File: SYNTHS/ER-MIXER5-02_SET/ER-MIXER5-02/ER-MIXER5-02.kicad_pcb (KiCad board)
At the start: 2 copper layers, 28 x 111.5 mm, 30 parts, among them J1 PJ-398SM, J2 PJ-398SM, J3 PJ-398SM, J4 PJ-398SM, J5 PJ-398SM, J6 PJ-398SM, J8 Conn_02x05, U1 TL072

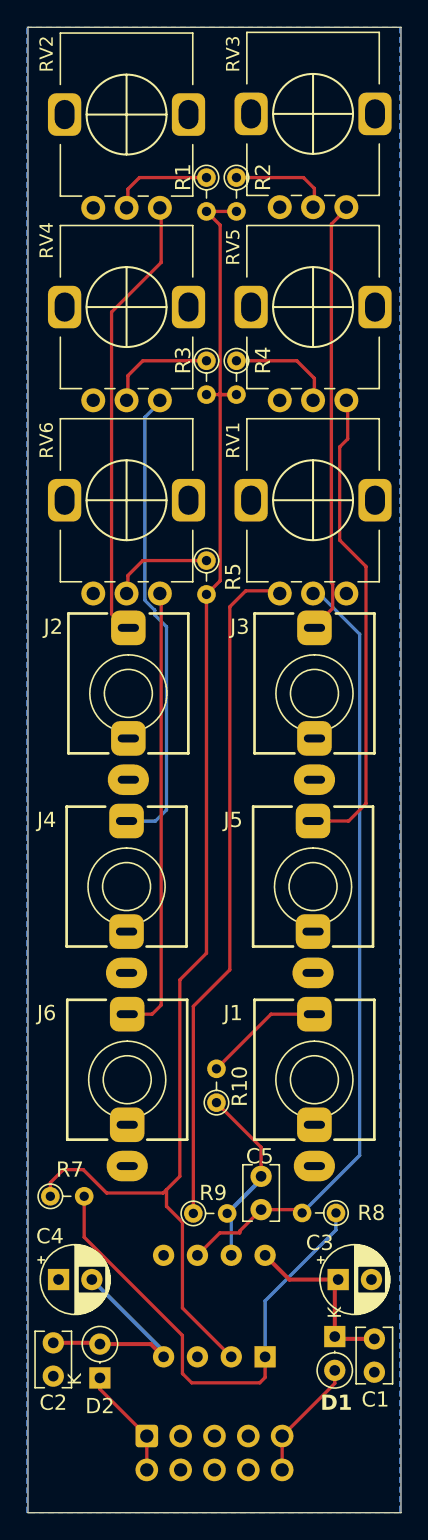
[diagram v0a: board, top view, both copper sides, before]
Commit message: cards
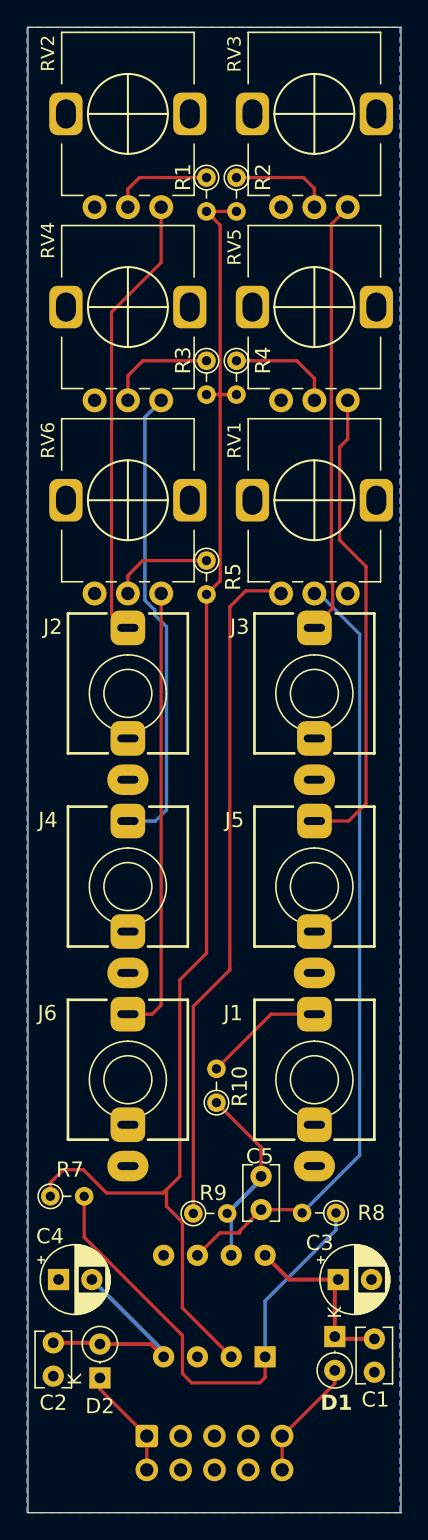
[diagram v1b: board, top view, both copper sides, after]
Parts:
- moved RV2 0.11 mm to (8.60, 15.0)
- moved J5 0.10 mm to (22.6, 73.0)
- moved RV1 0.10 mm to (22.6, 44.0)
- moved RV3 0.10 mm to (22.6, 15.0)
- moved RV5 0.10 mm to (22.6, 29.5)
- moved J4 0.10 mm to (8.60, 73.0)
- moved RV4 0.10 mm to (8.60, 29.5)
- moved RV6 0.10 mm to (8.60, 44.0)
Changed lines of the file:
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@@
   (net 23 "Net-(D2-K)")
   (footprint "LandBoards_Conns:RV09ACF" (layer "F.Cu")
-    (at 22.5 29.5 90)
+    (at 22.6 29.5 90)
     (descr "Potentiometer, vertical, Bourns PTV09A-1 Single, http://www.bourns.com/docs/Product-Datasheets/ptv09.pdf")
     (tags "Potentiometer vertical Bourns PTV09A-1 Single")
@@
   )
   (footprint "LandBoards_Conns:RV09ACF" (layer "F.Cu")
-    (at 22.5 44 90)
+    (at 22.6 44 90)
     (descr "Potentiometer, vertical, Bourns PTV09A-1 Single, http://www.bourns.com/docs/Product-Datasheets/ptv09.pdf")
     (tags "Potentiometer vertical Bourns PTV09A-1 Single")
@@
   )
   (footprint "LandBoards_Conns:RV09ACF" (layer "F.Cu")
-    (at 22.5 15 90)
+    (at 22.6 15 90)
     (descr "Potentiometer, vertical, Bourns PTV09A-1 Single, http://www.bourns.com/docs/Product-Datasheets/ptv09.pdf")
     (tags "Potentiometer vertical Bourns PTV09A-1 Single")
@@
   )
   (footprint "LandBoards_Conns:RV09ACF" (layer "F.Cu")
-    (at 8.5 44 90)
+    (at 8.6 44 90)
     (descr "Potentiometer, vertical, Bourns PTV09A-1 Single, http://www.bourns.com/docs/Product-Datasheets/ptv09.pdf")
     (tags "Potentiometer vertical Bourns PTV09A-1 Single")
@@
   )
   (footprint "AudioJacks:Jack_3.5mm_QingPu_WQP-PJ398SM_Vertical" (layer "F.Cu")
-    (at 22.5 73)
+    (at 22.6 73)
     (descr "T-S-SN Vertical mount jack AKA WQP-WQP518MA or Thonkiconn")
     (tags "WQP-WQP518MA, Thonkiconn")
@@
   )
   (footprint "AudioJacks:Jack_3.5mm_QingPu_WQP-PJ398SM_Vertical" (layer "F.Cu")
-    (at 8.55 87.5)
+    (at 8.6 87.5)
     (descr "T-S-SN Vertical mount jack AKA WQP-WQP518MA or Thonkiconn")
     (tags "WQP-WQP518MA, Thonkiconn")
@@
   )
   (footprint "AudioJacks:Jack_3.5mm_QingPu_WQP-PJ398SM_Vertical" (layer "F.Cu")
-    (at 8.636 58.5)
+    (at 8.6 58.5)
     (descr "T-S-SN Vertical mount jack AKA WQP-WQP518MA or Thonkiconn")
     (tags "WQP-WQP518MA, Thonkiconn")
@@
   )
   (footprint "AudioJacks:Jack_3.5mm_QingPu_WQP-PJ398SM_Vertical" (layer "F.Cu")
-    (at 8.5 73)
+    (at 8.6 73)
     (descr "T-S-SN Vertical mount jack AKA WQP-WQP518MA or Thonkiconn")
     (tags "WQP-WQP518MA, Thonkiconn")
@@
   )
   (footprint "LandBoards_Conns:RV09ACF" (layer "F.Cu")
-    (at 8.5 15.05 90)
+    (at 8.6 15 90)
     (descr "Potentiometer, vertical, Bourns PTV09A-1 Single, http://www.bourns.com/docs/Product-Datasheets/ptv09.pdf")
     (tags "Potentiometer vertical Bourns PTV09A-1 Single")
@@
   )
   (footprint "LandBoards_Conns:RV09ACF" (layer "F.Cu")
-    (at 8.5 29.5 90)
+    (at 8.6 29.5 90)
     (descr "Potentiometer, vertical, Bourns PTV09A-1 Single, http://www.bourns.com/docs/Product-Datasheets/ptv09.pdf")
     (tags "Potentiometer vertical Bourns PTV09A-1 Single")
@@
   )
   (footprint "AudioJacks:Jack_3.5mm_QingPu_WQP-PJ398SM_Vertical" (layer "F.Cu")
-    (at 22.606 58.5)
+    (at 22.6 58.5)
     (descr "T-S-SN Vertical mount jack AKA WQP-WQP518MA or Thonkiconn")
     (tags "WQP-WQP518MA, Thonkiconn")
